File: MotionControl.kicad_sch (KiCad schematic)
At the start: 26 parts, among them J15 Conn_01x05_Pin, J2 Conn_ARM_JTAG_SWD_10, Q1 2N7002, SW1 SW_Push, U1 ATSAMD21J18A-A, U7 TC4427, Y1 32.768kHz

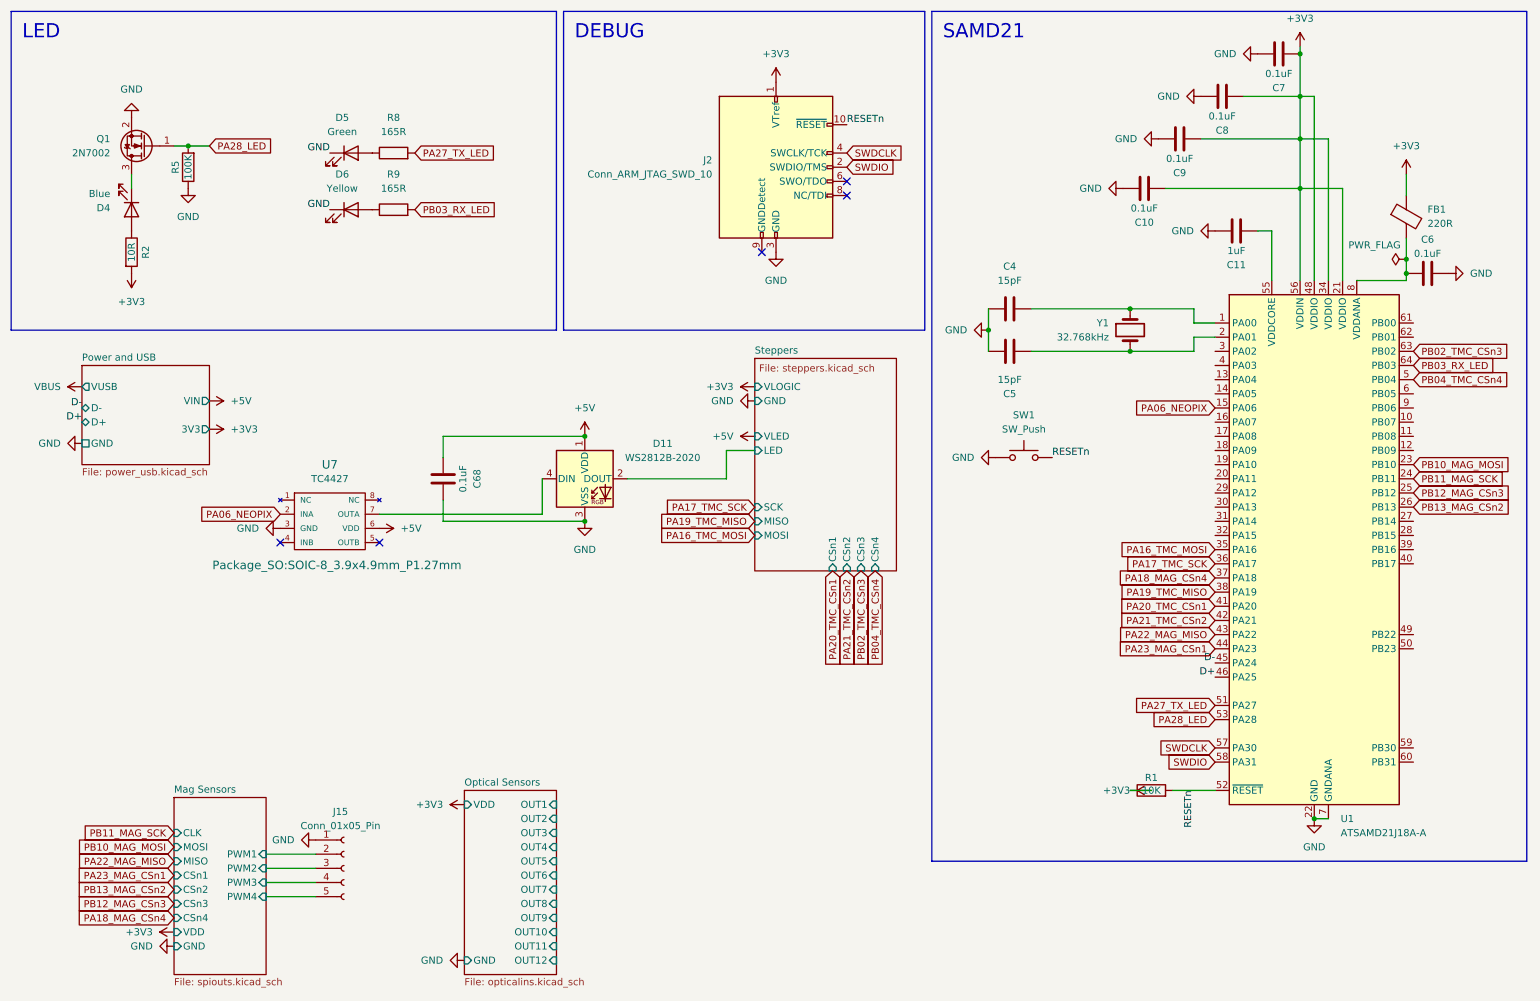
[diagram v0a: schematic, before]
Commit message: cs routing changes, endstop stuff
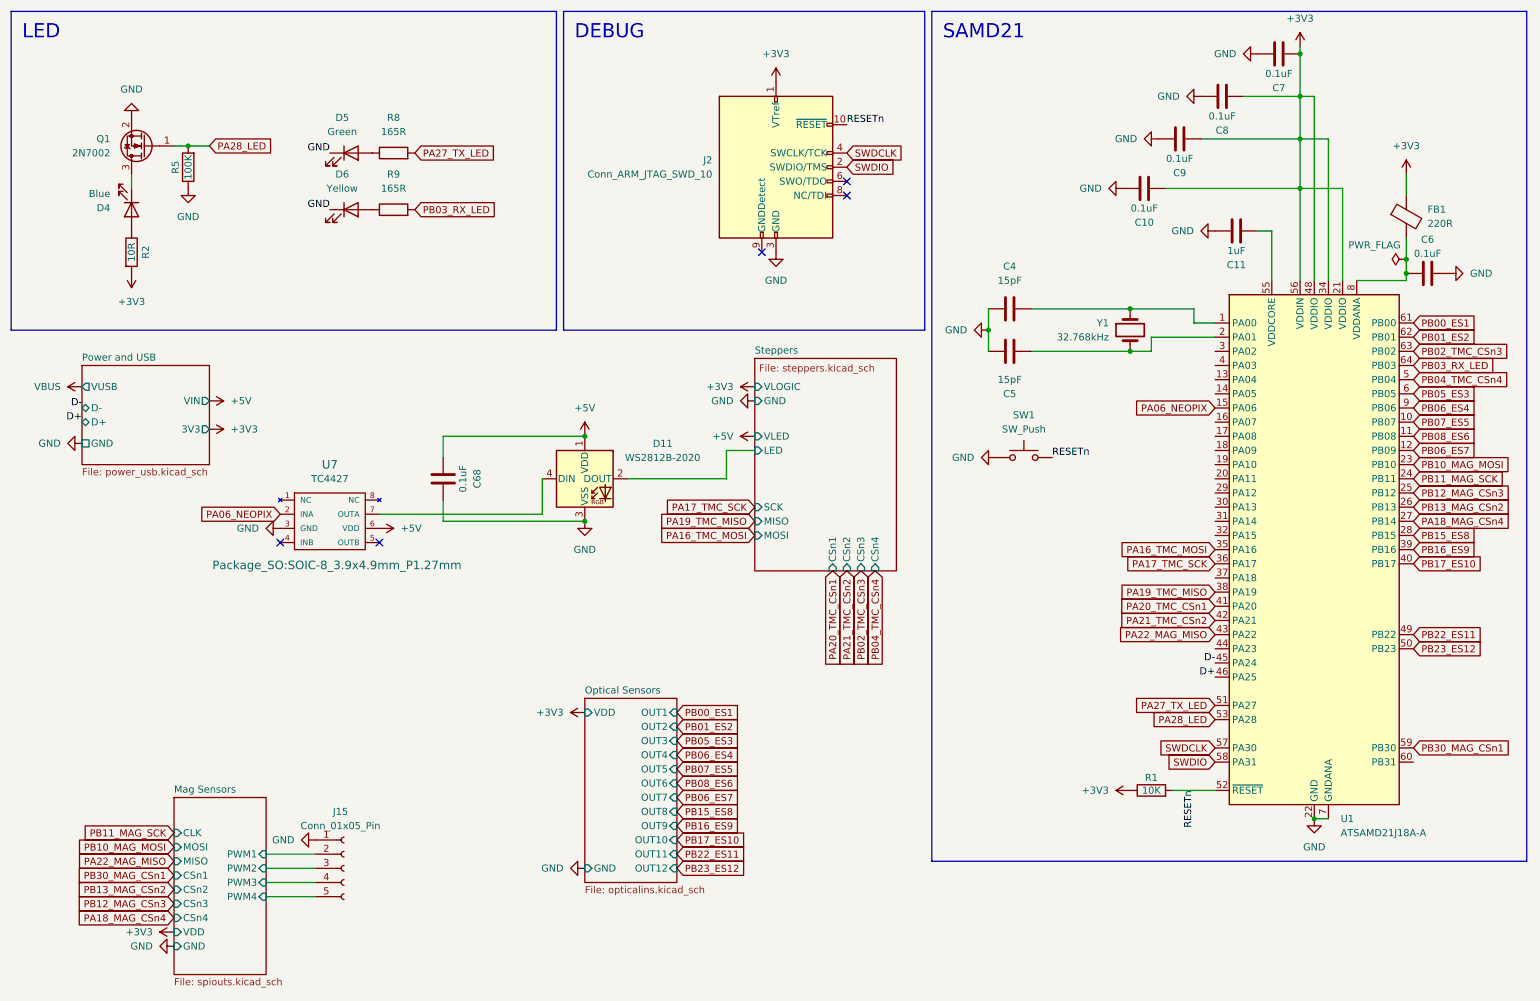
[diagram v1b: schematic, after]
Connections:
- net PA18_MAG_CSn4: now also U1.27 (PB14); no longer U1.37 (PA18)
- net PB07_ES5: now reaches U1.10 (PB07)
- net PB08_ES6: now reaches U1.11 (PB08)
- net PB06_ES7: now reaches U1.12 (PB09)
- net PB15_ES8: now reaches U1.28 (PB15)
- net PB16_ES9: now reaches U1.39 (PB16)
- net PB17_ES10: now reaches U1.40 (PB17)
- net PB22_ES11: now reaches U1.49 (PB22)
- net PB23_ES12: now reaches U1.50 (PB23)
- net PB30_MAG_CSn1: now reaches U1.59 (PB30)
- net PB05_ES3: now reaches U1.6 (PB05)
- net PB00_ES1: now reaches U1.61 (PB00)
- net PB01_ES2: now reaches U1.62 (PB01)
- net PB06_ES4: now reaches U1.9 (PB06)
- net PA23_MAG_CSn1: no longer names the net of U1.44 (PA23)
